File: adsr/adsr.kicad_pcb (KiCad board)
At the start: 2 copper layers, 80.3 x 112.3 mm, 41 parts, among them J10 Conn_01x08_Male, J11 Conn_01x08_Female, J12 Conn_01x08_Male, J3 B_IN, J4 A_IN, J5 B_OUT, J6 A_OUT, J7 EURORACK_CONN_16, J8 Conn_01x04_Male, J9 Conn_01x08_Female, Q1 2N3904, Q2 2N3904, Q5 DMMT5401, U1 LM13700, U2 TL074, U3 DG403, U4 DG403

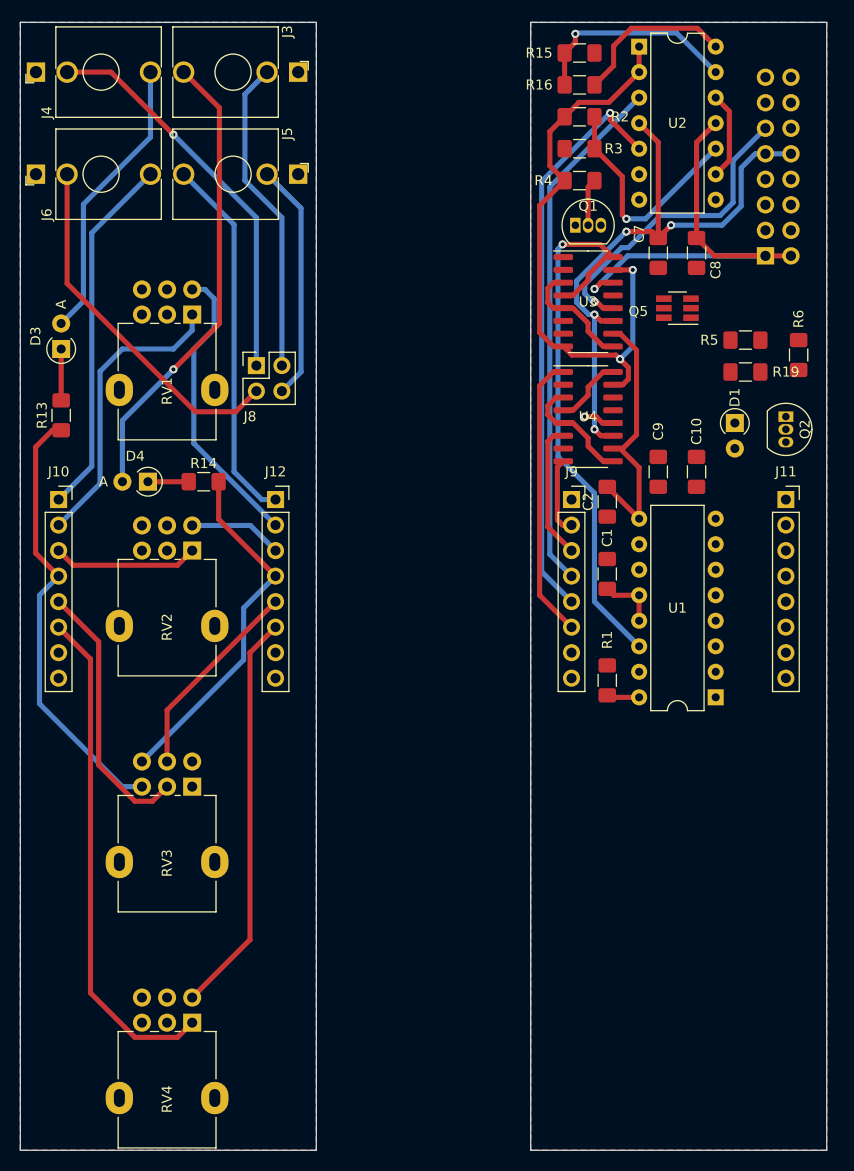
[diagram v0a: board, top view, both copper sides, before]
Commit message: layout
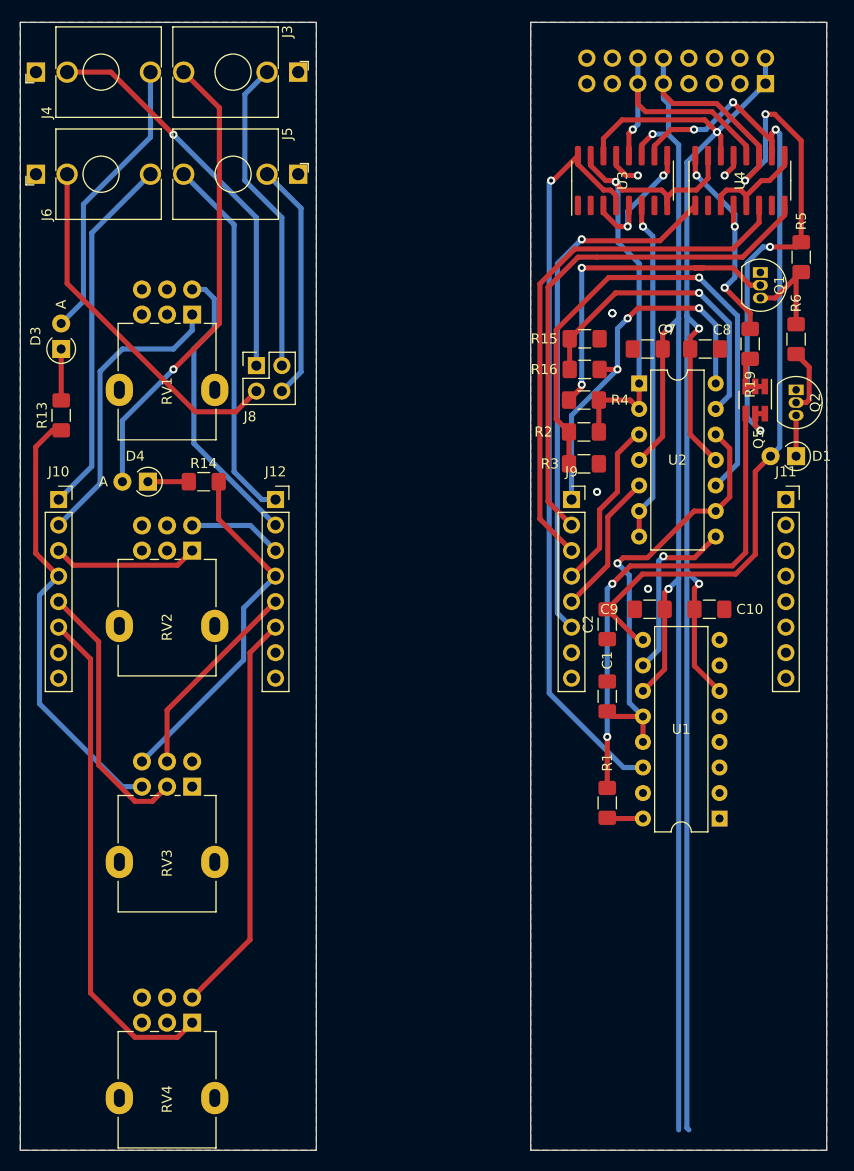
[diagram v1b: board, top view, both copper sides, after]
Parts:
- moved U2 33.5 mm to (76.8, 53.2)
- moved R2 31.4 mm to (71.3, 58.0), turned to 180 degrees
- moved R3 31.4 mm to (71.3, 61.2), turned to 0 degrees
- moved R15 28.5 mm to (71.4, 48.8)
- moved R16 28.3 mm to (71.4, 51.8)
- moved U4 27.9 mm to (86.9, 33.0), turned to 90 degrees
- moved R4 21.8 mm to (71.3, 54.9), turned to 180 degrees
- moved Q1 19.0 mm to (88.9, 42.2), turned to 270 degrees
- moved J7 17.1 mm to (89.4, 23.4), turned to 90 degrees
- moved C10 13.7 mm to (83.8, 75.7), turned to 180 degrees
- moved C9 13.7 mm to (77.9, 75.7), turned to 180 degrees
- moved U3 12.5 mm to (75.2, 33.0), turned to 90 degrees
- moved C1 12.2 mm to (73.7, 84.4)
- moved C2 12.2 mm to (73.7, 77.2)
- moved R1 12.2 mm to (73.7, 95.0)
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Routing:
- net +12V: track 61.8 -> 205.6 mm, vias 4 -> 7
- net -12V: track 42.8 -> 156.8 mm, vias 1 -> 3
- net /envelope/STATE: track 27.3 -> 85.6 mm, vias 0 -> 3
- net Net-(Q5-Pad4): track 0.00 -> 48.9 mm, vias 0 -> 2
- net /envelope/ATTACK: track 37.1 -> 82.4 mm
- net /envelope/SUS_RAW: track 84.3 -> 41.2 mm, vias 1 -> 0
- net /envelope/DECAY: track 28.1 -> 68.4 mm
- net /envelope/REF_RAW: track 96.3 -> 61.2 mm
- net /envelope/SUS: track 0.00 -> 34.0 mm, vias 0 -> 1
- net Net-(R2-Pad2): track 23.3 -> 53.4 mm
- net Net-(C1-Pad1): track 14.7 -> 43.3 mm, vias 0 -> 1
- net Net-(Q1-Pad2): track 4.71 -> 33.1 mm, vias 0 -> 2
- net /envelope/RELEASE: track 78.5 -> 103.3 mm, vias 0 -> 1
- net A_OUT: track 52.5 -> 74.0 mm, vias 0 -> 3
- net Net-(U1-Pad14): track 55.9 -> 74.1 mm
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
